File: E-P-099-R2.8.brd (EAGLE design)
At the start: 100 x 80 mm, 86 parts, among them J1 AVR_ISP

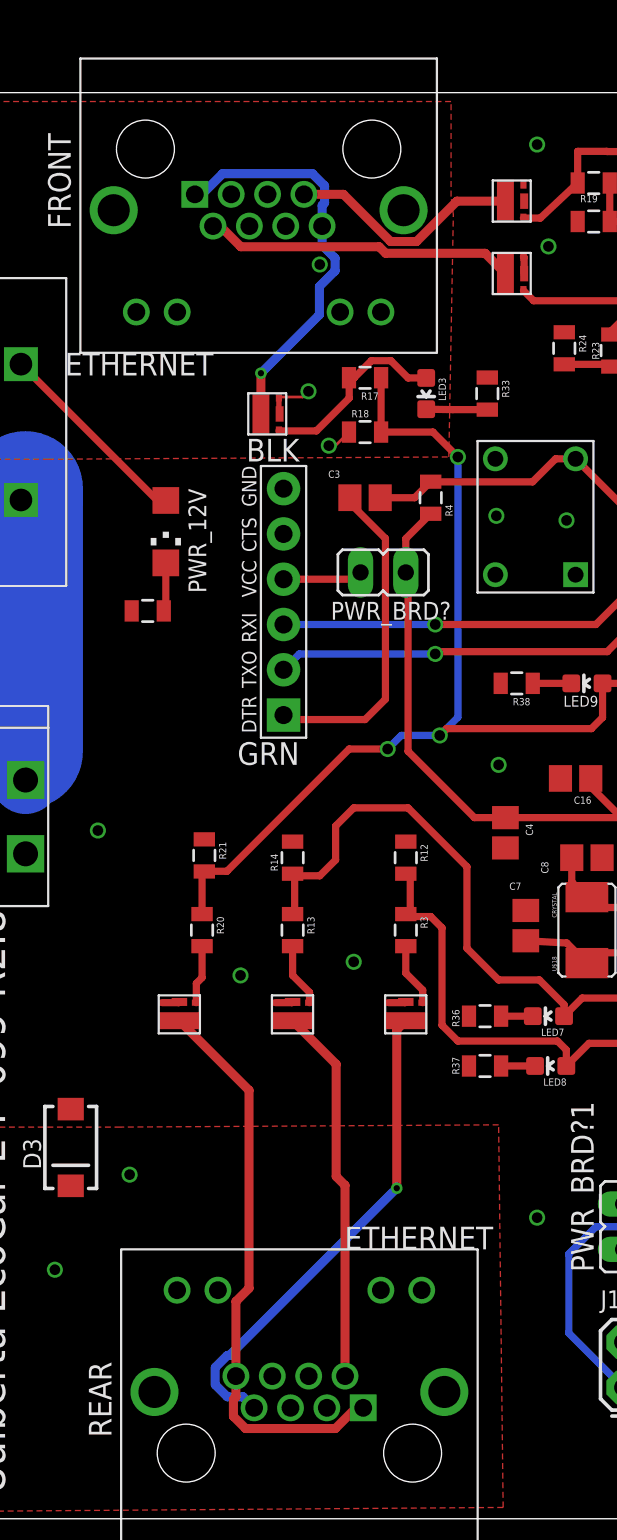
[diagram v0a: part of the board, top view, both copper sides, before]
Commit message: Revert "pinouts updated to match new light boards"
This reverts commit c6705fe930e627c4a8d5c034fe7450b97c4f4bb6.
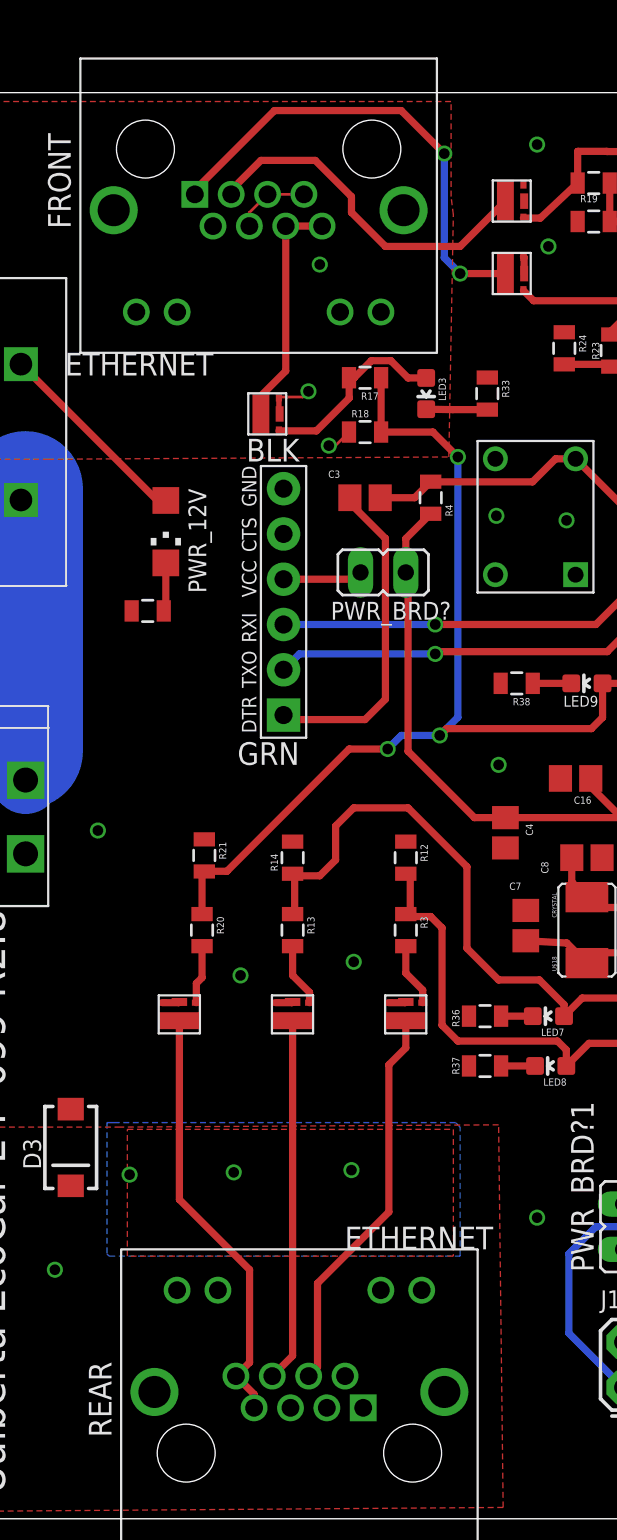
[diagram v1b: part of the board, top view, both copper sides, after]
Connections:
- removed net N$14: FRONT.P$2, U$20.D
- removed net N$15: FRONT.P$7, U$11.D
- new net N$20: FRONT.P$1, U$20.D
- new net N$23: FRONT.P$3, U$11.D
- net +12V: now also FRONT.P$2, FRONT.P$7, REAR.P$1, REAR.P$2; no longer FRONT.P$3, FRONT.P$6, REAR.P$4, REAR.P$6
- net N$27: now also FRONT.P$6; no longer FRONT.P$1
- net N$4: now also REAR.P$7; no longer REAR.P$1
- net N$43: now also REAR.P$4; no longer REAR.P$7
- net N$5: now also REAR.P$6; no longer REAR.P$2
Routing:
- net N$20: track 0.00 -> 26.7 mm, vias 0 -> 2
- net N$23: track 0.00 -> 19.9 mm
- net N$14: track 17.5 -> 0.00 mm
- net N$15: track 13.3 -> 0.00 mm
- net N$27: track 23.9 -> 13.2 mm, vias 1 -> 0
- net N$4: track 32.2 -> 24.1 mm
- net N$43: track 27.6 -> 22.2 mm, vias 1 -> 0
- net +12V: track 11.3 -> 15.6 mm, vias 1 -> 3
- net N$5: track 21.2 -> 20.4 mm
- added copper zone on layer 16, net +12V

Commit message: pinouts updated to match new light boards
New changes to the pinouts for the ethernet connectors to match the new design of the head and tail light boards. Also designed to be symmetric across the connector to prevent mistakes.
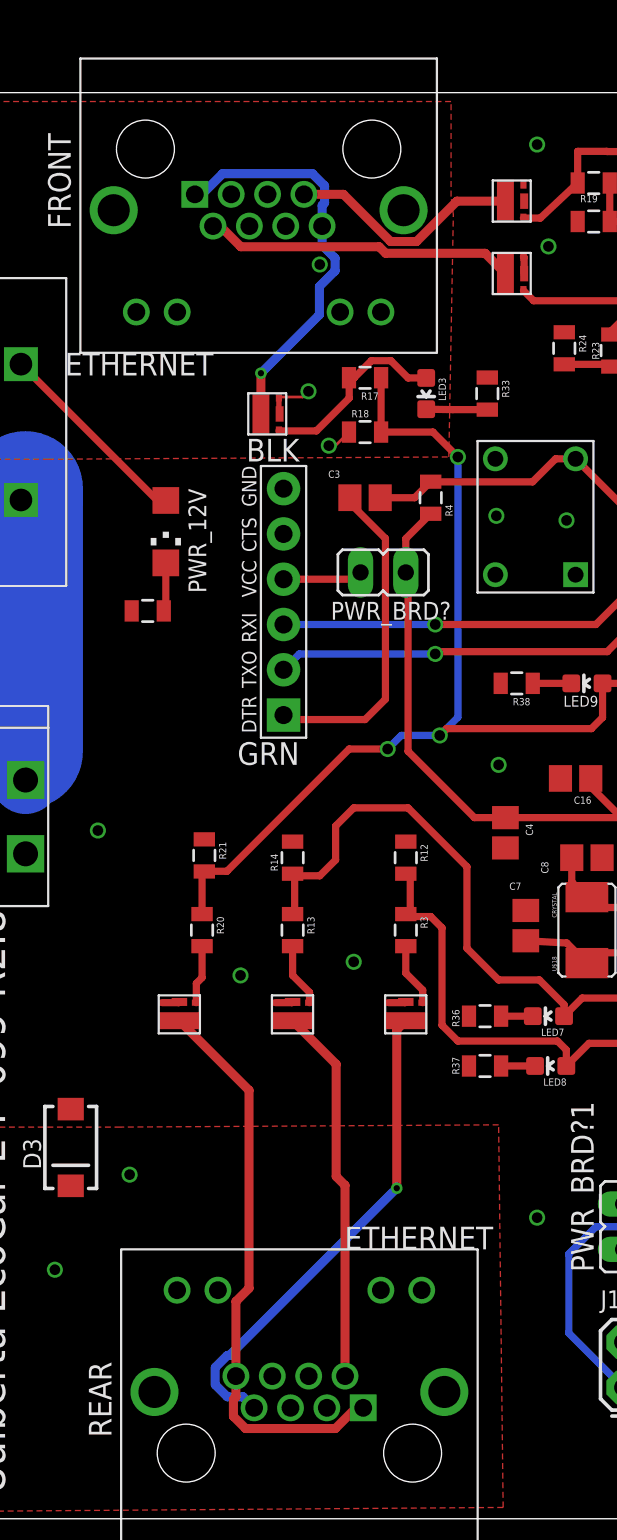
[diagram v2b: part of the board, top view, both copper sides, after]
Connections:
- removed net N$20: FRONT.P$1, U$20.D
- removed net N$23: FRONT.P$3, U$11.D
- new net N$14: FRONT.P$2, U$20.D
- new net N$15: FRONT.P$7, U$11.D
- net +12V: now also FRONT.P$3, FRONT.P$6, REAR.P$4, REAR.P$6; no longer FRONT.P$2, FRONT.P$7, REAR.P$1, REAR.P$2
- net N$27: now also FRONT.P$1; no longer FRONT.P$6
- net N$4: now also REAR.P$1; no longer REAR.P$7
- net N$43: now also REAR.P$7; no longer REAR.P$4
- net N$5: now also REAR.P$2; no longer REAR.P$6
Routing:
- net N$20: track 26.7 -> 0.00 mm, vias 2 -> 0
- net N$23: track 19.9 -> 0.00 mm
- net N$14: track 0.00 -> 17.5 mm
- net N$15: track 0.00 -> 13.3 mm
- net N$27: track 13.2 -> 23.9 mm, vias 0 -> 1
- net N$4: track 24.1 -> 32.2 mm
- net N$43: track 22.2 -> 27.6 mm, vias 0 -> 1
- net +12V: track 15.6 -> 11.3 mm, vias 3 -> 1
- net N$5: track 20.4 -> 21.2 mm
- removed copper zone on layer 16, net +12V
